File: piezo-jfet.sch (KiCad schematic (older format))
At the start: 25 parts, among them J1 XLR3, J2 Conn_01x01_Female, J3 Conn_01x01_Female, J4 Conn_01x01_Female, J5 Conn_01x01_Female, J6 Conn_01x01_Female, Q1 J105, Q2 LSK389B, X1 XTAL, X2 XTAL

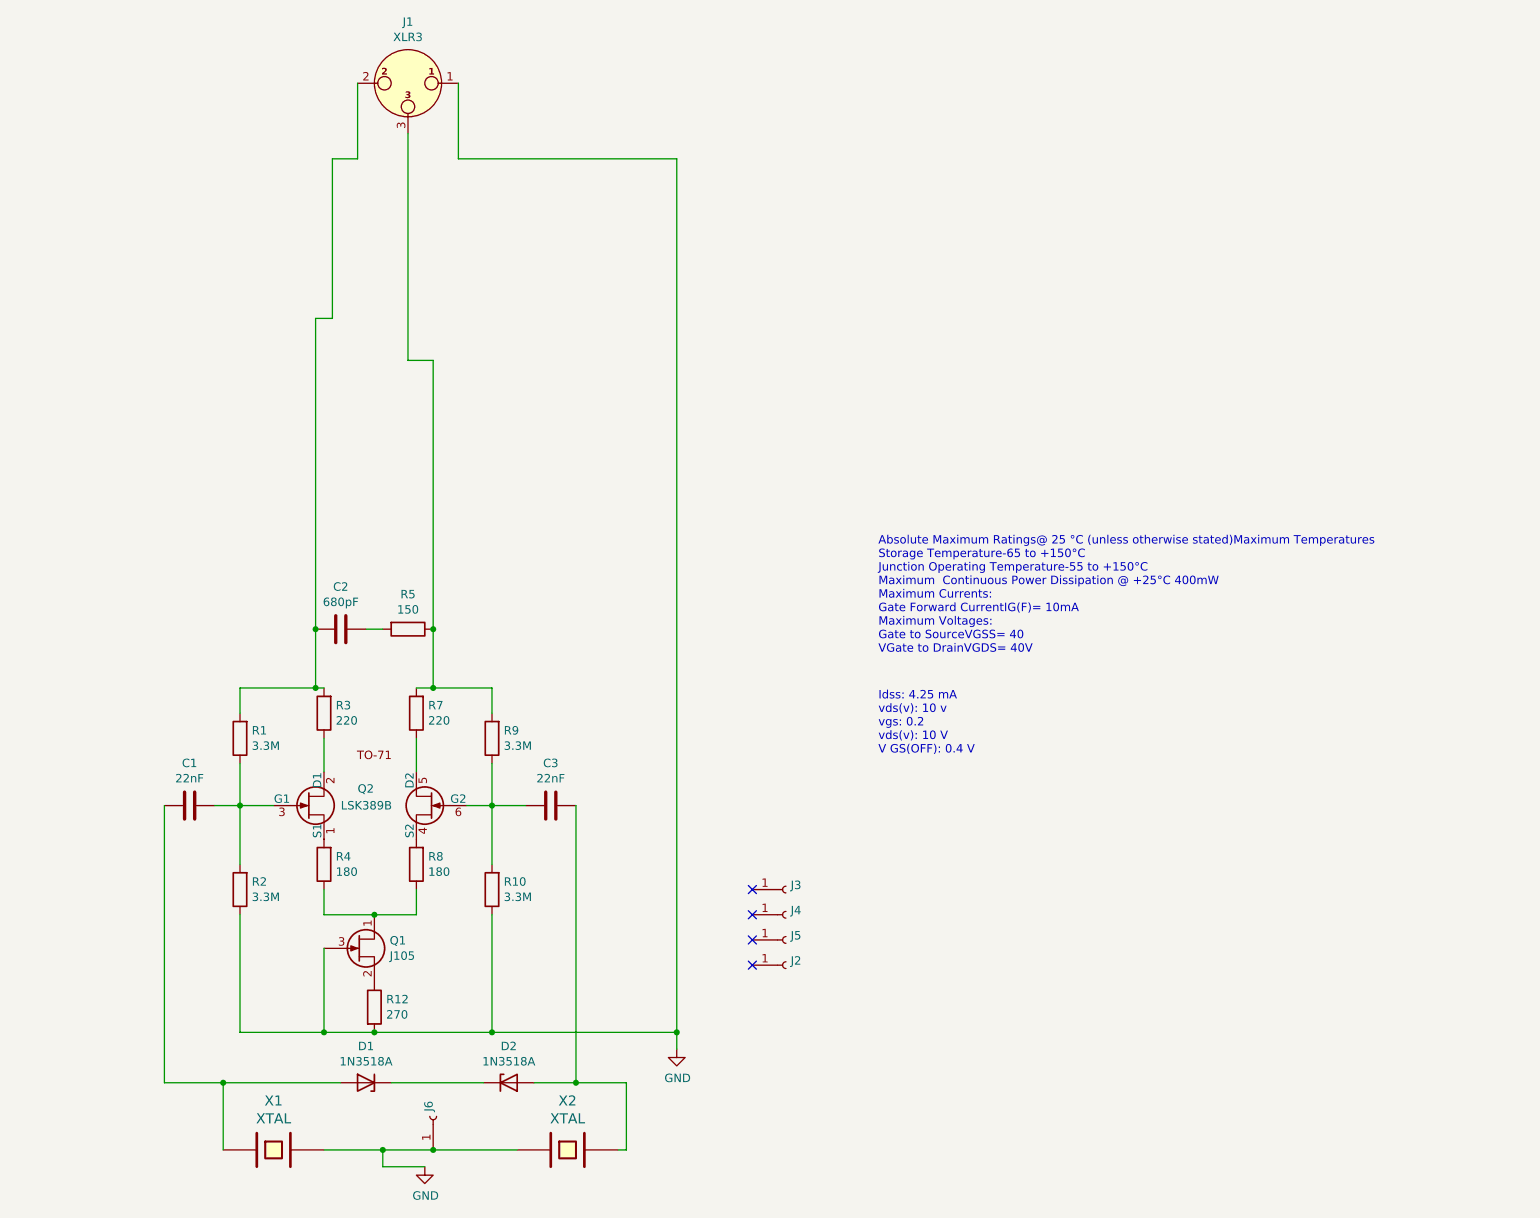
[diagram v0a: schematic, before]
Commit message: updated files
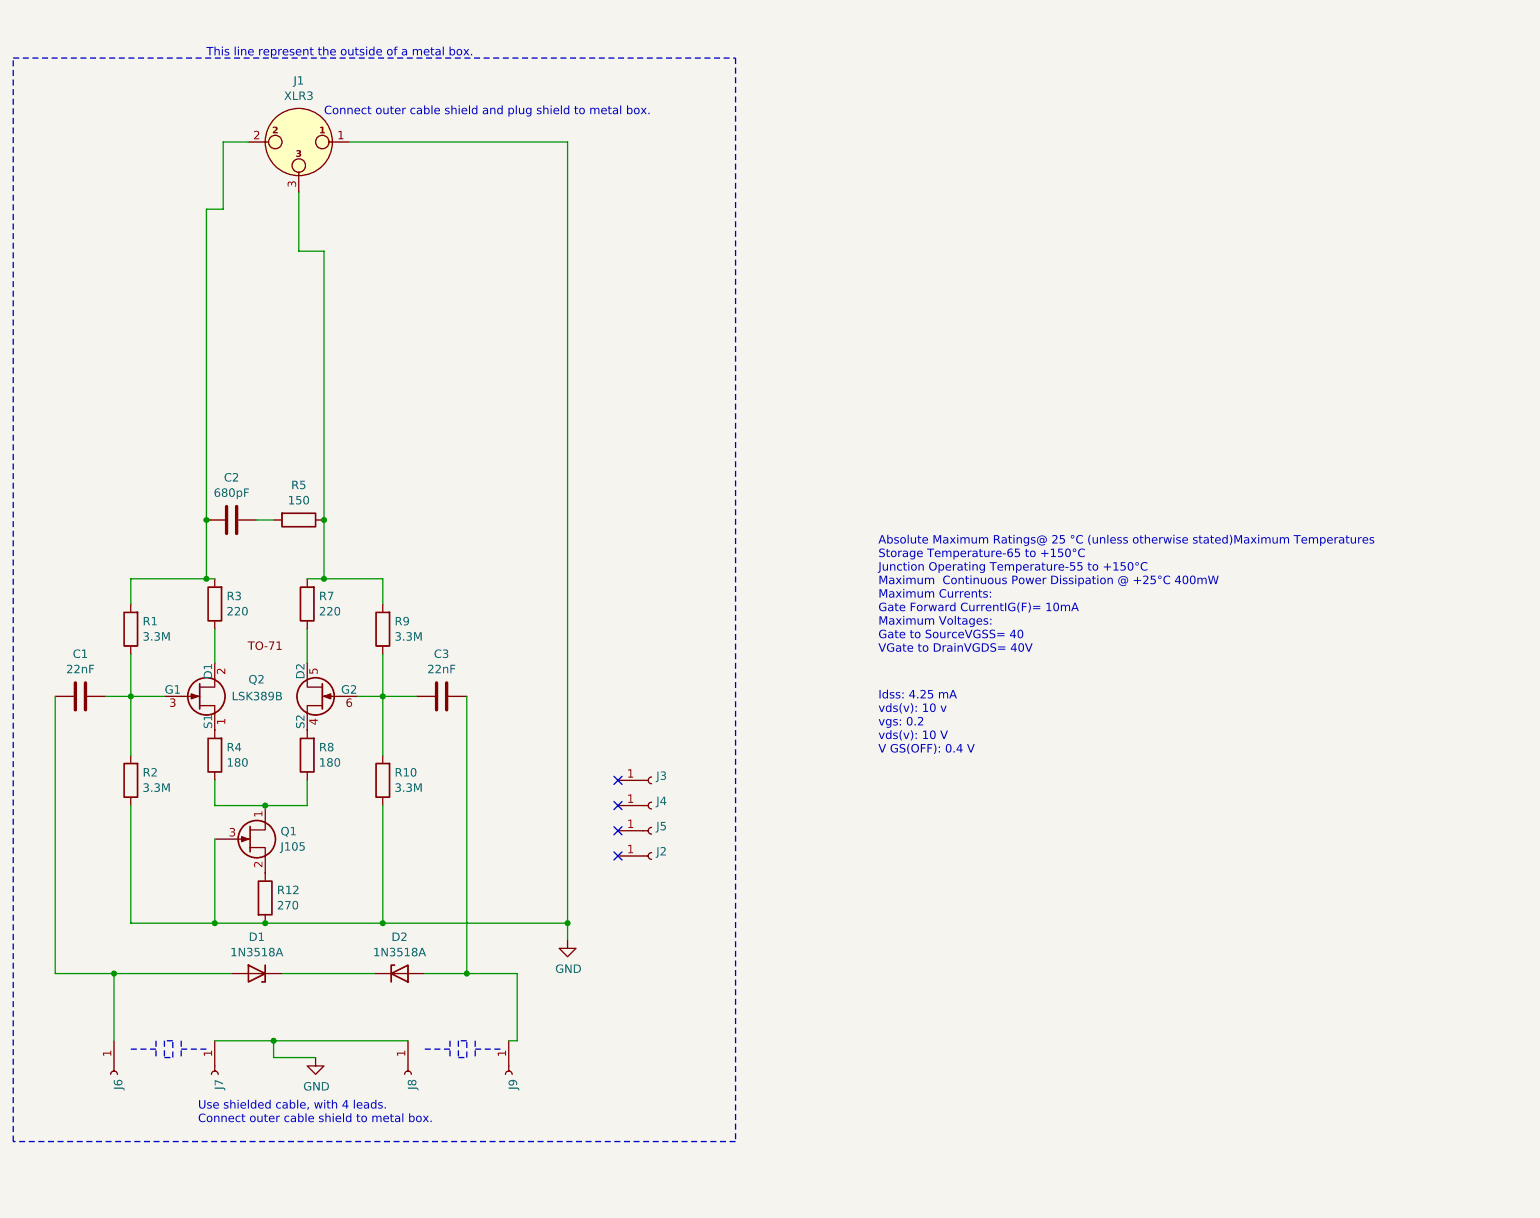
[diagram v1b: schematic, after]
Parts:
- removed X1, X2: XTAL, Connector_PinSocket_2.54mm:PinSocket_1x02_P2.54mm_Vertical, symbol piezo-jfet-rescue:XTAL-Keyboard
- added J7, J8, J9: Conn_01x01_Female, MountingHole:MountingHole_2.2mm_M2_DIN965_Pad, symbol Connector:Conn_01x01_Female
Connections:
- net GND: now also J7.1 (Pin_1), J8.1 (Pin_1); no longer J6.1 (Pin_1)
- net at C1.2, D1.2 (A): now also J6.1 (Pin_1)
- net at C3.1, D2.2 (A): now also J9.1 (Pin_1)
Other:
- note added: "Connect outer cable shield and plug shield to metal box."
- note added: "This line represent the outside of a metal box."
- note added: "Use shielded cable, with 4 leads.\nConnect outer cable shield to metal box."
- moved on the sheet: C1, C2, C3, D1, D2, J1, J2, J3, J4, J5, Q1, Q2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
